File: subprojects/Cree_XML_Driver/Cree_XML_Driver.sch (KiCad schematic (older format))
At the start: 58 parts, among them J101 PJ-102AH, J102 Conn_01x03, Q101 Si2302CDS-T1, Q102 Si2302CDS-T1, Q103 Si2302CDS-T1, Q104 Si2302CDS-T1, U101 PAM2804, U102 PAM2804, U103 PAM2804, U104 PAM2804, U105 WS2811, U106 74HC14D,653, U107 WS2811

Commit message: Led horiz
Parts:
- TP101: footprint TestPoint:TestPoint_THTPad_2.0x2.0mm_Drill1.0mm -> TestPoint:TestPoint_THTPad_1.0x1.0mm_Drill0.5mm
- U105, U107: footprint Package_SO:SO-8_3.9x4.9mm_P1.27mm -> Package_SO:SOIC-8_3.9x4.9mm_P1.27mm

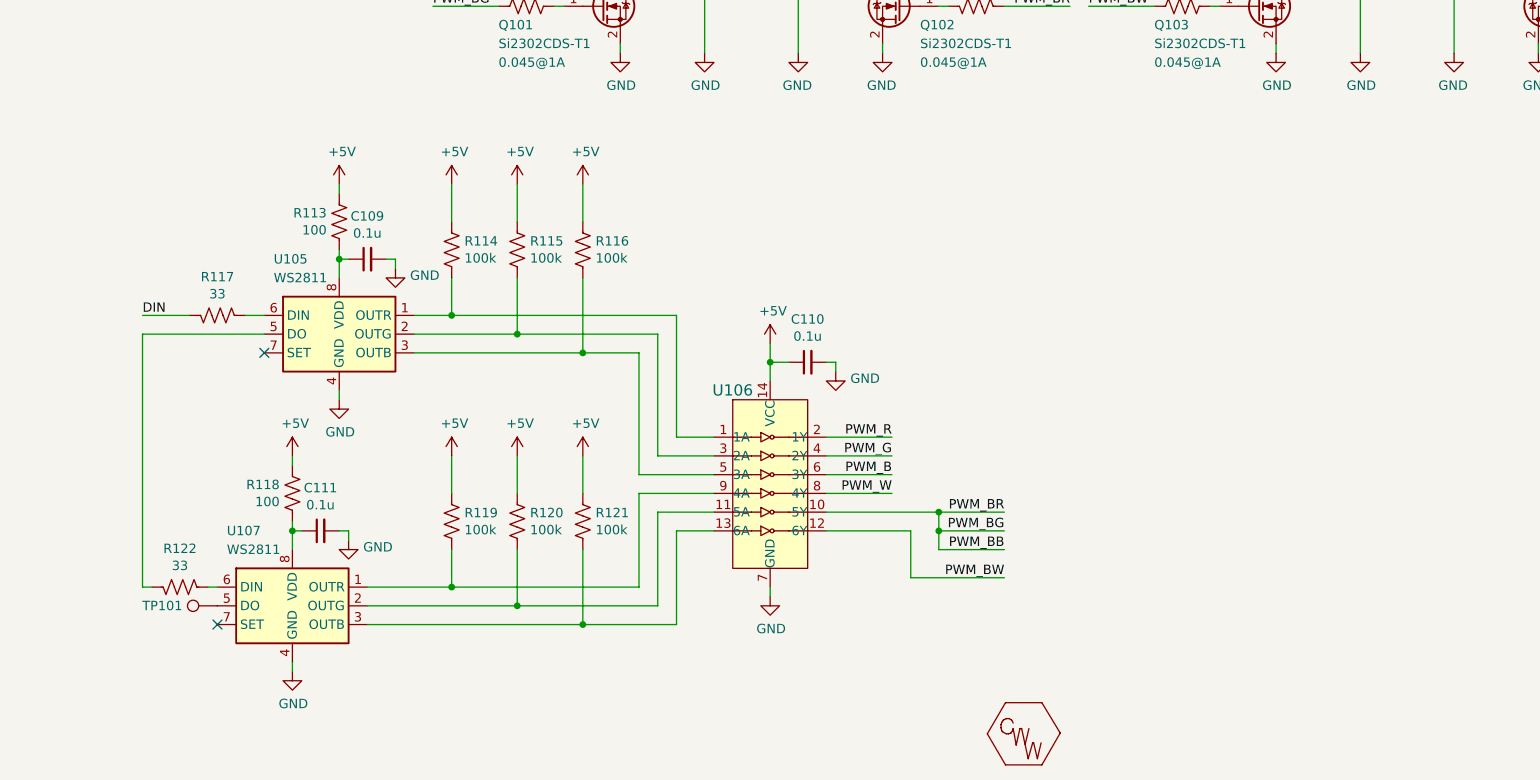
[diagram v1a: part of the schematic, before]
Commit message: Finish up led
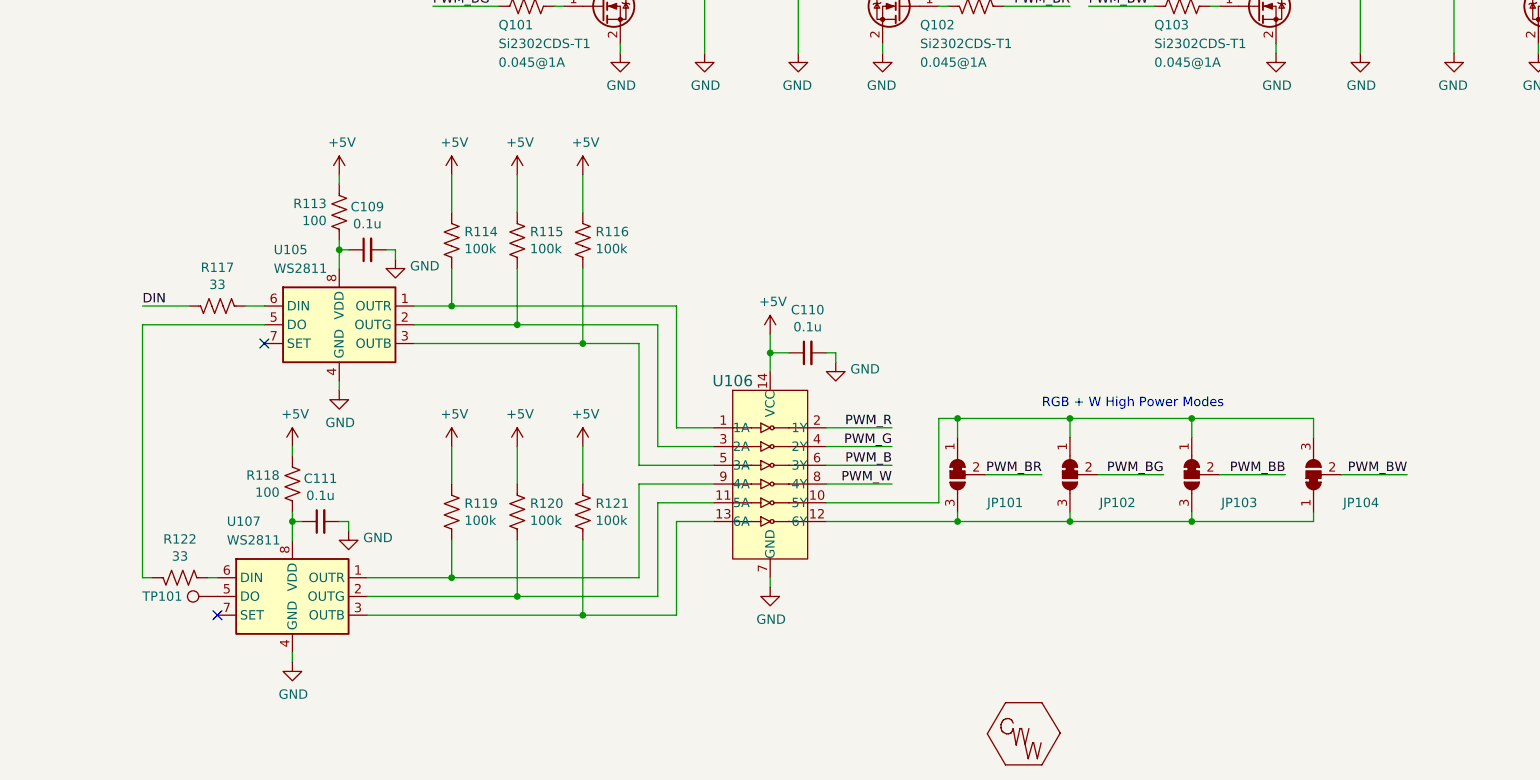
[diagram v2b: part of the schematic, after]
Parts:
- added JP101, JP102, JP103, JP104: SolderJumper_3_Bridged12, Jumper:SolderJumper-3_P1.3mm_Bridged12_Pad1.0x1.5mm, symbol Jumper:SolderJumper_3_Bridged12
- J102: footprint Connector_PinSocket_1.27mm:PinSocket_1x03_P1.27mm_Vertical -> Connector_PinHeader_2.54mm:PinHeader_1x03_P2.54mm_Horizontal
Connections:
- net PWM_BB: now also JP103.2 (C); no longer R109.2, R110.2, U106.10 (5Y)
- net PWM_BW: now also JP104.2 (C); no longer U106.12 (6Y)
- new net: JP101.1 (A), JP102.1 (A), JP103.1 (A), JP104.3 (B), U106.10 (5Y)
- new net: JP101.3 (B), JP102.3 (B), JP103.3 (B), JP104.1 (A), U106.12 (6Y)
- new net PWM_BG: JP102.2 (C), R109.2
- new net PWM_BR: JP101.2 (C), R110.2
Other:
- note added: "RGB + W High Power Modes"
- moved on the sheet: C109, C110, C111, R113, R114, R115, R116, R117, R118, R119, R120, R121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
